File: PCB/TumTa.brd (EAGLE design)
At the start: 16 parts

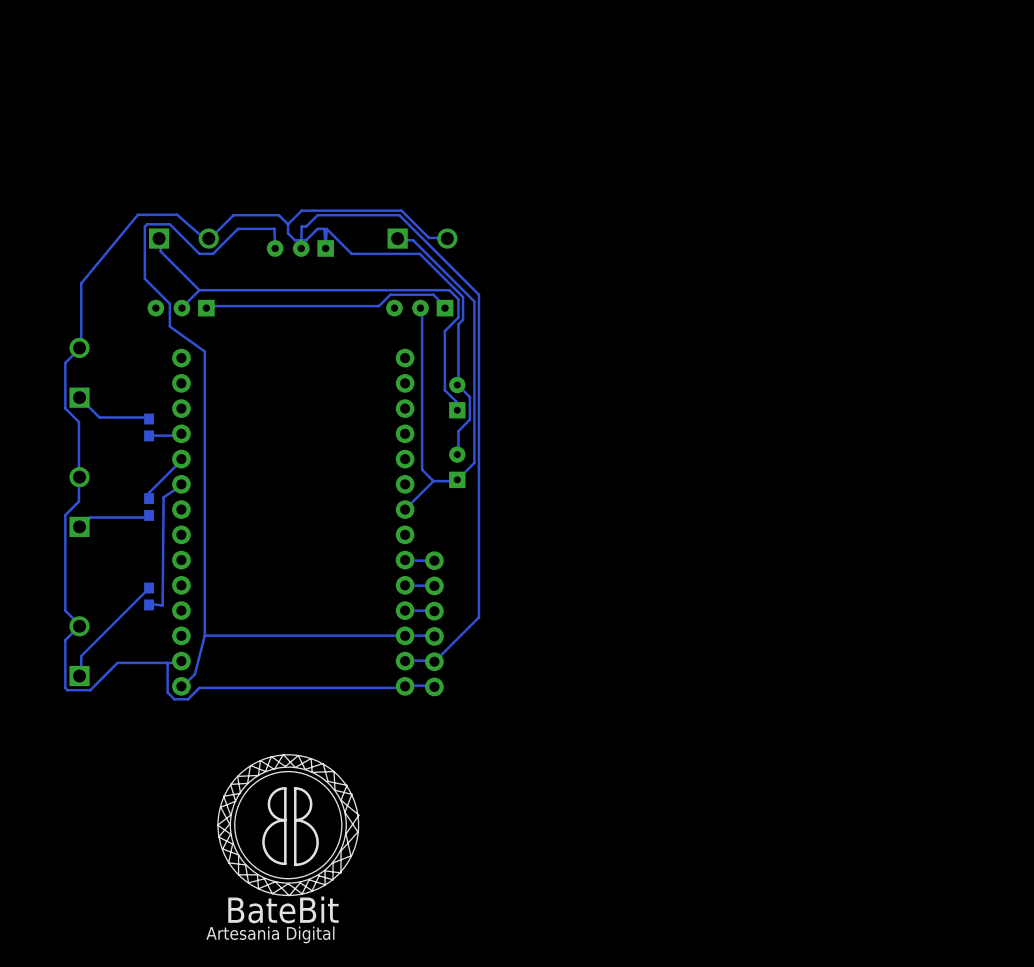
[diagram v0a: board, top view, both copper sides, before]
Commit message: v0_2_4
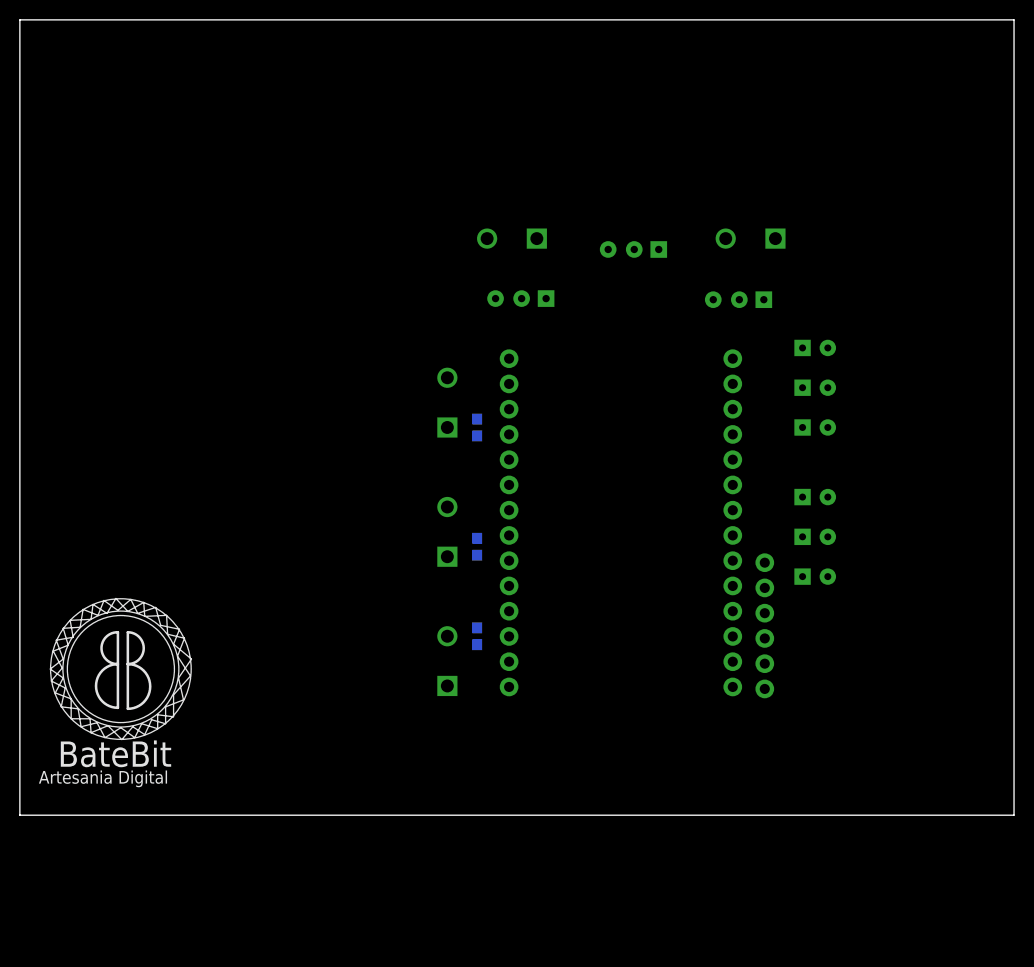
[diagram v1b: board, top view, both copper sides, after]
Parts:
- added C3, C4, C5, C6: (no value), SparkFun-Passives:CPOL-RADIAL-10UF-25V
- moved TA 62.0 mm to (76.0, 58.0), turned to 0 degrees
- moved CAL_TA 56.1 mm to (77.1, 49.9)
- moved C2 38.6 mm to (80.0, 28.0), turned to 0 degrees
- moved LED1(VERDE) 37.1 mm to (43.0, 26.0)
- moved LED2(AMARELO) 37.1 mm to (43.0, 39.0)
- moved SWITCH_STANDBY 37.0 mm to (43.0, 13.0)
- moved C1 36.1 mm to (80.0, 32.0), turned to 0 degrees
- moved CAL_TETO 33.5 mm to (66.5, 54.9)
- moved R1 33.2 mm to (46.0, 27.0)
- moved R4 33.2 mm to (46.0, 18.0), turned to 90 degrees
- moved JP1 33.2 mm to (74.9, 25.4)
- moved R2 33.0 mm to (46.0, 39.0)
- moved FIO_SHIELD 33.0 mm to (61.0, 27.9)
- moved FL1 23.0 mm to (10.2, 12.7)
- moved TUM 14.0 mm to (52.0, 58.0), turned to 0 degrees
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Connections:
- net N$4 renamed D9
- net N$5 renamed D10
- removed net 3.3V: CAL_TA.1, CAL_TUM.1
- removed net N$1: FIO_SHIELD.9, R4.2
- removed net N$11: FIO_SHIELD.24
- removed net N$12: C2.1, CAL_TA.2, TA.1
- removed net N$9: C1.1, CAL_TUM.2, FIO_SHIELD.22, TUM.1
- new net A0: C1.1, C2.1, C3.1, CAL_TUM.2, FIO_SHIELD.21, TUM.1
- new net A1: C4.1, C5.1, C6.1, CAL_TA.2, FIO_SHIELD.22, TA.1
- new net D6: FIO_SHIELD.7, R4.2
- net 3V3: now also CAL_TA.1, CAL_TUM.1
- net GND: now also C3.2, C4.2, C5.2, C6.2
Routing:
- net GND: track 174.6 -> 0.00 mm
- net 3V3: track 90.3 -> 0.00 mm
- net AREF: track 65.6 -> 0.00 mm
- net N$9: track 53.5 -> 0.00 mm
- net N$12: track 48.1 -> 0.00 mm
- net 3.3V: track 25.2 -> 0.00 mm
- net N$1: track 14.6 -> 0.00 mm
- net N$2: track 11.7 -> 0.00 mm
- net N$7: track 7.88 -> 0.00 mm
- net N$3: track 7.47 -> 0.00 mm
- net D9: track 5.30 -> 0.00 mm
- net D10: track 3.43 -> 0.00 mm
- net RXI: track 2.96 -> 0.00 mm
- net DTR: track 2.96 -> 0.00 mm
- net TXO: track 2.96 -> 0.00 mm
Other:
- board outline added: 100 x 80 mm
